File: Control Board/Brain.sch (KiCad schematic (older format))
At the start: 36 parts, among them J10 USB_B_Micro, J11 Conn_ARM_JTAG_SWD_10, J9 Conn_ARM_JTAG_SWD_10, SW2 SW_Push, U1 ATSAMD21G18A-AU, U6 AT24C32, Y1 32768Hz

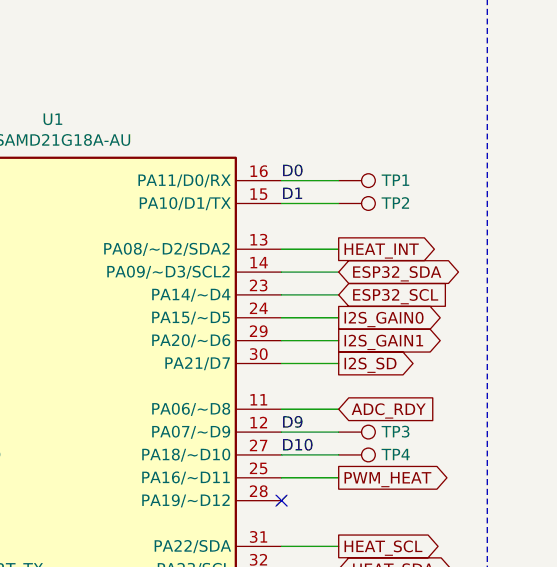
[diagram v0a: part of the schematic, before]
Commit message: Start of V2.1 PCB.
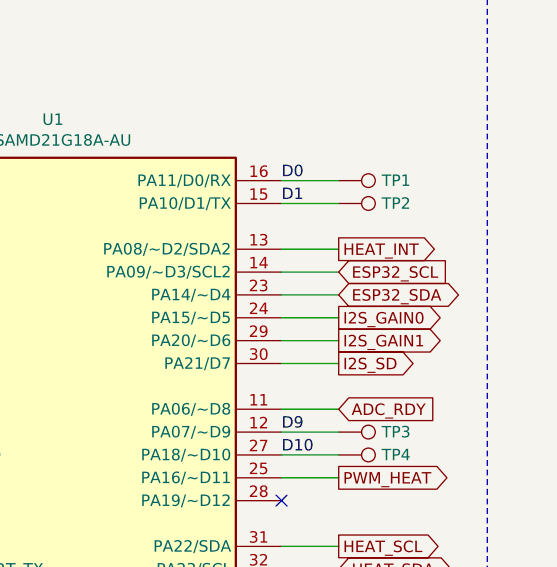
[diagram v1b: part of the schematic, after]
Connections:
- net ESP32_SCL: now also U1.14 (PA09/~~D3/SCL2); no longer U1.23 (PA14/~~D4)
- net ESP32_SDA: now also U1.23 (PA14/~~D4); no longer U1.14 (PA09/~~D3/SCL2)
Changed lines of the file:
@@
 Sheet 4 5
 Title "IoT12-hardware brain"
-Date "2021-02-22"
-Rev "V2.0"
+Date "2021-03-07"
+Rev "V2.1"
 Comp ""
 Comment1 ""
@@
 	0    -1   -1   0
 $EndComp
-Text GLabel 10500 2000 2    50   BiDi ~ 0
+Text GLabel 10500 2100 2    50   BiDi ~ 0
 ESP32_SDA
 Wire Wire Line
@@
 Text Notes 600  5500 0    118  ~ 0
 The pull is strong
-Text GLabel 10500 2100 2    50   Input ~ 0
+Text GLabel 10500 2000 2    50   Input ~ 0
 ESP32_SCL
 Wire Notes Line
